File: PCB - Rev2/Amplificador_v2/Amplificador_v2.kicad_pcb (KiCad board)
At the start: 2 copper layers, 150 x 100 mm, 156 parts, among them IC1 AD817, IC2 AD817, J1 Conector alimentacion, J2 Conector alimentacion, J3 Conn_01x02_Male, J4 Conn_01x03_Male, J5 Conn_01x03_Male, J6 Screw_Terminal_01x02, J7 Conn_01x02_Male, J8 Conn_01x03_Male, J9 Screw_Terminal_01x03, Q1 BC847, Q10 BC847, Q11 BC857, Q12 BC847, Q13 2N7002, Q14 BC847, Q15 BC857, Q16 PHB27NQ10T, Q17 PHB27NQ10T, Q2 BC847, Q3 BC847, Q4 2N7002, Q5 BC857, Q6 BC847, Q7 BC847, Q8 BC857, Q9 BC857, U1 TL082, U10 LM7805_TO220, U2 LM311, U3 LM311, U4 SN74LVC2G02DCUR, U5 LM311, U6 UCC20520DWR, U7 LM7812_TO220, U8 LM7815_TO220, U9 LM7915_TO220

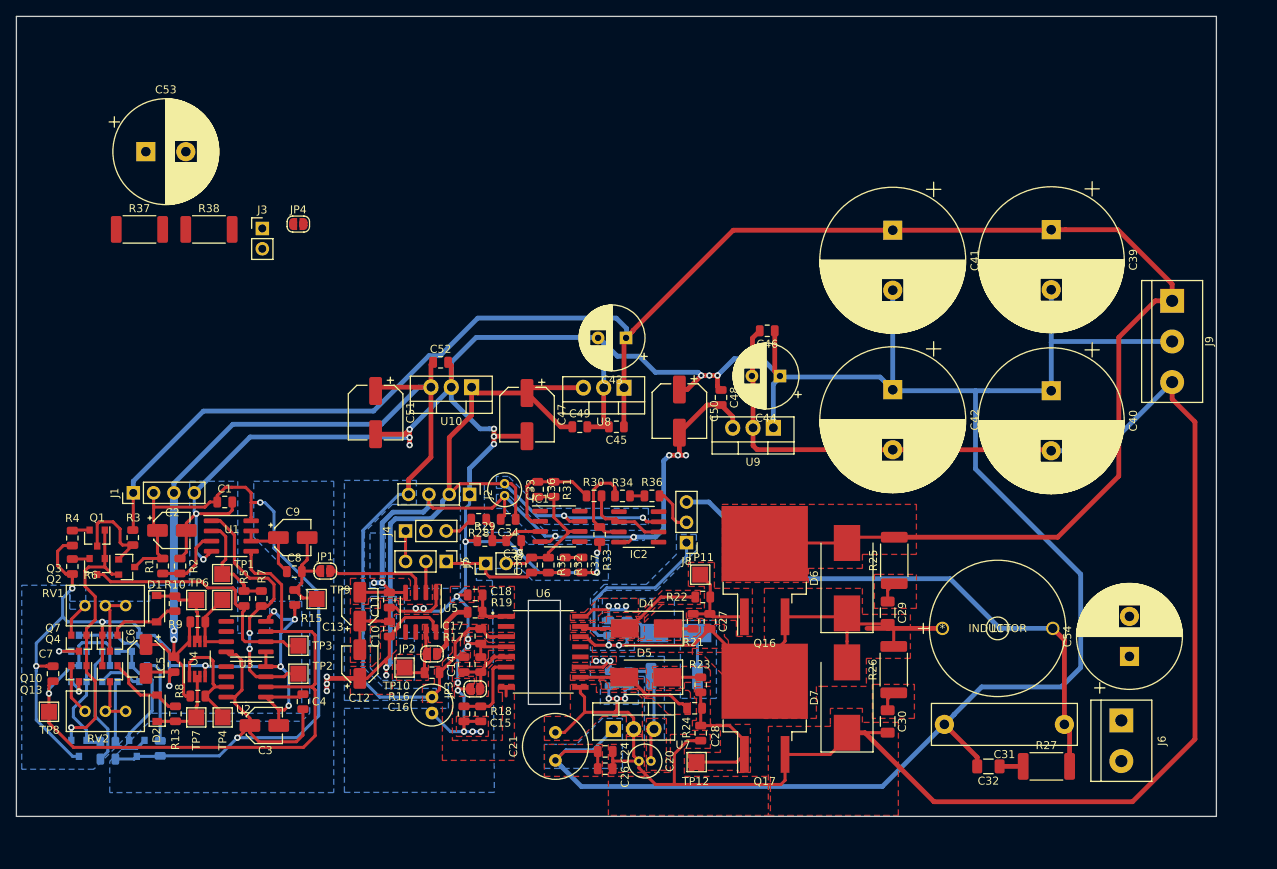
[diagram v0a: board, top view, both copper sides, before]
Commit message: Finalizada la placa v2
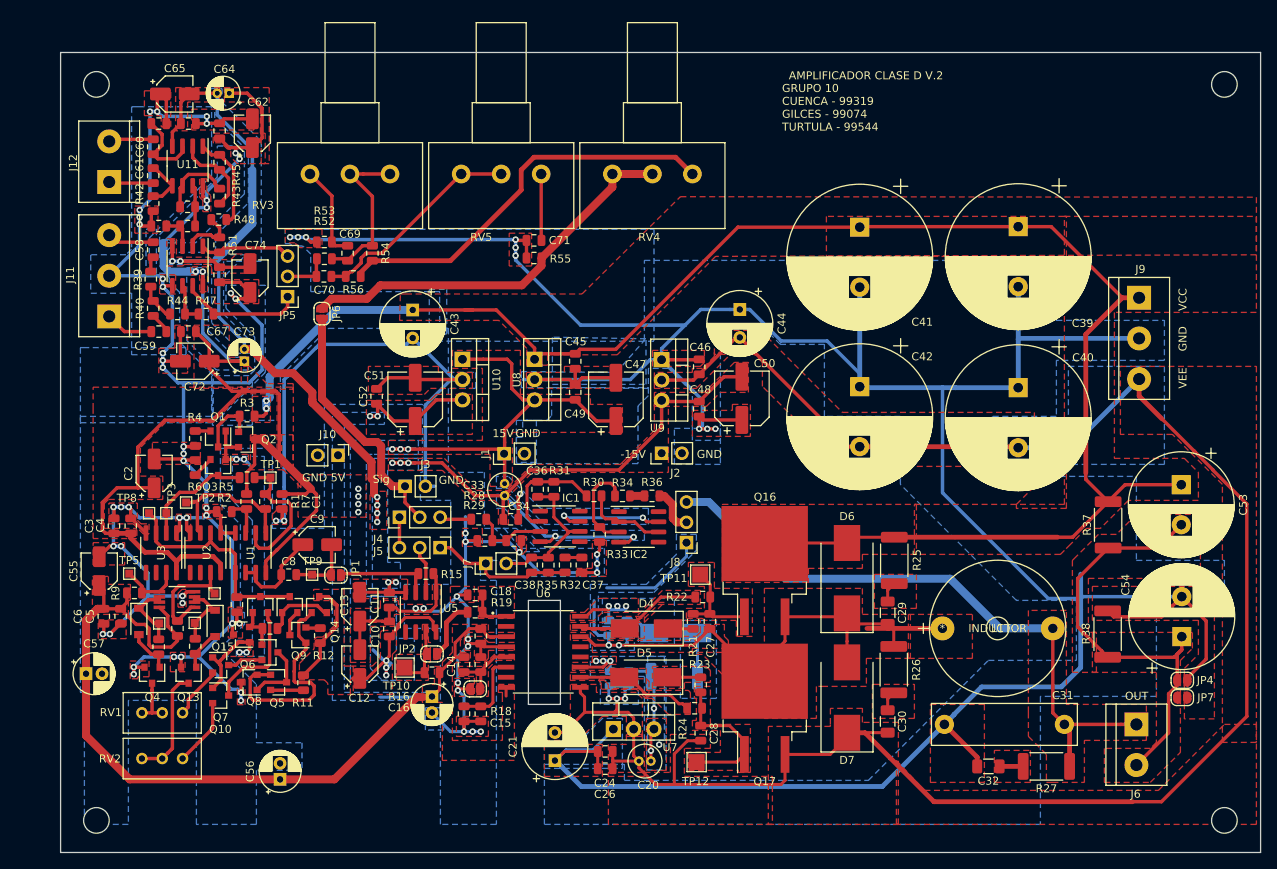
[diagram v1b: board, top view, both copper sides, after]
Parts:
- added C55: 10u, Capacitor_SMD:CP_Elec_4x5.3, F.Cu at (50.4, 144.3)
- added C56: 10u, Capacitor_THT:CP_Radial_D5.0mm_P2.00mm, F.Cu at (73.0, 170.4)
- added C57: 10u, Capacitor_THT:CP_Radial_D5.0mm_P2.00mm, F.Cu at (48.7, 157.2)
- added C58: C, Capacitor_SMD:C_0805_2012Metric, F.Cu at (57.1, 104.2)
- added C59: C, Capacitor_SMD:C_0805_2012Metric, F.Cu at (57.8, 114.4)
- added C60: C, Capacitor_SMD:C_0805_2012Metric, F.Cu at (57.1, 91.3)
- added C61: C, Capacitor_SMD:C_0805_2012Metric, F.Cu at (57.1, 94.9)
- added C62: 10u, Capacitor_SMD:CP_Elec_4x5.3, F.Cu at (69.5, 89.6)
- added C63: C, Capacitor_SMD:C_0805_2012Metric, F.Cu at (65.4, 89.3)
- added C64: 10u, Capacitor_THT:CP_Radial_D4.0mm_P1.50mm, F.Cu at (66.6, 84.6)
- added C65: 10u, Capacitor_SMD:CP_Elec_4x5.3, F.Cu at (59.8, 84.7)
- added C66: C, Capacitor_SMD:C_0805_2012Metric, F.Cu at (61.5, 88.4)
- added C67: C, Capacitor_SMD:C_0805_2012Metric, F.Cu at (61.5, 114.4)
- added C68: C, Capacitor_SMD:C_0805_2012Metric, F.Cu at (65.4, 107.3)
- added C69: C, Capacitor_SMD:C_0805_2012Metric, F.Cu at (81.4, 104.6)
- added C70: C, Capacitor_SMD:C_0805_2012Metric, F.Cu at (78.4, 107.5)
- added C71: C, Capacitor_SMD:C_0805_2012Metric, F.Cu at (104.7, 103.0)
- added C72: 10u, Capacitor_SMD:CP_Elec_4x5.3, F.Cu at (62.3, 118.1)
- added C73: 10u, Capacitor_THT:CP_Radial_D4.0mm_P1.50mm, F.Cu at (68.5, 118.1)
- added C74: 10u, Capacitor_SMD:CP_Elec_4x5.3, F.Cu at (69.2, 107.7)
- added J10: Conn_01x02_Male, Connector_PinHeader_2.54mm:PinHeader_1x02_P2.54mm_Vertical, F.Cu at (80.2, 129.9)
- added J11: Screw_Terminal_01x03, TerminalBlock:TerminalBlock_bornier-3_P5.08mm, F.Cu at (51.6, 112.5)
- added J12: Screw_Terminal_01x02, TerminalBlock:TerminalBlock_bornier-2_P5.08mm, F.Cu at (51.6, 95.7)
- added JP5: Jumper_3_Open, Connector_PinHeader_2.54mm:PinHeader_1x03_P2.54mm_Vertical, F.Cu at (73.9, 110.0)
- added JP6: Jumper_Preampli, Jumper:SolderJumper-2_P1.3mm_Open_RoundedPad1.0x1.5mm, F.Cu at (78.2, 112.2)
- added JP7: Jumper, Jumper:SolderJumper-2_P1.3mm_Open_RoundedPad1.0x1.5mm, F.Cu at (185.7, 160.1)
- added R39: R, Resistor_SMD:R_0805_2012Metric, F.Cu at (56.8, 107.8)
- added R40: R, Resistor_SMD:R_0805_2012Metric, F.Cu at (57.1, 111.5)
- added R41: R, Resistor_SMD:R_0805_2012Metric, F.Cu at (57.8, 88.4)
- added R42: R, Resistor_SMD:R_0805_2012Metric, F.Cu at (57.1, 98.4)
- added R43: R, Resistor_SMD:R_0805_2012Metric, F.Cu at (65.4, 97.5)
- added R44: R, Resistor_SMD:R_0805_2012Metric, F.Cu at (60.1, 112.2)
- added R45: R, Resistor_SMD:R_0805_2012Metric, F.Cu at (65.4, 93.2)
- added R46: R, Resistor_SMD:R_0805_2012Metric, F.Cu at (61.4, 98.8)
- added R47: R, Resistor_SMD:R_0805_2012Metric, F.Cu at (63.7, 112.2)
- added R48: R, Resistor_SMD:R_0805_2012Metric, F.Cu at (65.3, 100.4)
- added R49: R, Resistor_SMD:R_0805_2012Metric, F.Cu at (61.4, 101.2)
- added R50: R, Resistor_SMD:R_0805_2012Metric, F.Cu at (57.8, 101.2)
- added R51: R, Resistor_SMD:R_0805_2012Metric, F.Cu at (65.4, 103.6)
- added R52: R, Resistor_SMD:R_0805_2012Metric, F.Cu at (78.5, 105.3)
- added R53: R, Resistor_SMD:R_0805_2012Metric, F.Cu at (78.5, 103.2)
- added R54: R, Resistor_SMD:R_0805_2012Metric, F.Cu at (84.5, 104.6)
- added R55: R, Resistor_SMD:R_0805_2012Metric, F.Cu at (104.7, 105.2)
- added R56: R, Resistor_SMD:R_0805_2012Metric, F.Cu at (82.1, 107.5)
- added REF**: MountingHole_3.2mm_M3, MountingHole:MountingHole_3.2mm_M3, F.Cu at (50.0, 175.5)
- added REF**: MountingHole_3.2mm_M3, MountingHole:MountingHole_3.2mm_M3, F.Cu at (191.0, 175.5)
- added REF**: MountingHole_3.2mm_M3, MountingHole:MountingHole_3.2mm_M3, F.Cu at (191.0, 83.5)
- added REF**: MountingHole_3.2mm_M3, MountingHole:MountingHole_3.2mm_M3, F.Cu at (50.0, 83.5)
- added RV3: R_POT, Potentiometer_THT:Potentiometer_Alps_RK163_Single_Horizontal, F.Cu at (86.7, 94.7)
- added RV4: R_POT, Potentiometer_THT:Potentiometer_Alps_RK163_Single_Horizontal, F.Cu at (124.5, 94.7)
- added RV5: R_POT, Potentiometer_THT:Potentiometer_Alps_RK163_Single_Horizontal, F.Cu at (105.6, 94.7)
- added U11: NE5532, Package_SO:SOIC-8_3.9x4.9mm_P1.27mm, F.Cu at (61.4, 93.7)
- added U12: NE5532, Package_SO:SOIC-8_3.9x4.9mm_P1.27mm, F.Cu at (61.4, 106.2)
- C16: footprint Capacitor_THT:C_Radial_D5.0mm_H11.0mm_P2.00mm -> Capacitor_THT:CP_Radial_D5.0mm_P2.00mm
- C21: footprint Capacitor_THT:C_Radial_D8.0mm_H11.5mm_P3.50mm -> Capacitor_THT:CP_Radial_D8.0mm_P3.50mm
- C3: value 10u -> 100n; footprint Capacitor_SMD:CP_Elec_4x5.3 -> Capacitor_SMD:C_0805_2012Metric
- C6: value 10u -> 220n; footprint Capacitor_SMD:CP_Elec_4x5.3 -> Capacitor_SMD:C_0805_2012Metric
- J1, J2: value Conector alimentacion -> Conn_01x02_Male; footprint Connector_PinHeader_2.54mm:PinHeader_1x04_P2.54mm_Vertical -> Connector_PinHeader_2.54mm:PinHeader_1x02_P2.54mm_Vertical
- Q11, Q12, Q14, Q15, Q5, Q6, Q8, Q9, R11, R12, R14: moved to F.Cu
- TP1, TP2, TP3, TP4, TP5, TP6, TP7, TP8, TP9: footprint TestPoint:TestPoint_Pad_2.0x2.0mm -> TestPoint:TestPoint_Pad_1.0x1.0mm
- moved C53 136.0 mm to (185.6, 133.5), turned to 270 degrees
- moved R37 126.6 mm to (176.5, 138.6), turned to 90 degrees
- moved JP4 124.3 mm to (185.7, 158.0), turned to 180 degrees
- moved R38 123.2 mm to (176.4, 152.2), turned to 270 degrees
- moved J1 46.6 mm to (101.0, 129.7)
- moved J3 36.8 mm to (88.6, 133.7), turned to 90 degrees
- moved C3 31.2 mm to (52.2, 138.7), turned to 90 degrees
- moved C4 30.8 mm to (54.3, 138.7)
- moved Q14 29.0 mm to (77.9, 148.5), turned to 90 degrees
- moved TP8 27.8 mm to (56.6, 137.1), turned to 270 degrees
- moved C43 26.9 mm to (89.5, 111.7), turned to 270 degrees
- moved R11 26.2 mm to (75.9, 158.3), turned to 270 degrees
- moved TP2 25.6 mm to (61.2, 135.8), turned to 270 degrees
- moved Q15 24.8 mm to (68.1, 152.3), turned to 180 degrees
- moved R14 24.8 mm to (71.7, 151.5)
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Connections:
- J1 pad 1: VCC -> +15V
- J1 pad 2: +15V -> GND
- J2 pad 1: GND -> -15V
- J2 pad 2: +15V -> GND
- R15 pad 1: Net-(C8-Pad2) -> Vtriang
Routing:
- net GND: track 603.4 -> 813.2 mm, vias 34 -> 67
- net -15V: track 90.4 -> 184.8 mm, vias 7 -> 13
- net /Vtriang_off: track 92.9 -> 28.1 mm, vias 1 -> 0
- net Net-(C53-Pad2): track 0.00 -> 55.8 mm
- net /Filter_out: track 0.00 -> 50.3 mm
- net Net-(JP6-Pad1): track 0.00 -> 49.8 mm
- net +15V: track 239.8 -> 279.2 mm, vias 9 -> 19
- net Signal_in: track 0.00 -> 31.7 mm
- net Net-(C70-Pad2): track 0.00 -> 26.9 mm
- net VCC: track 241.6 -> 217.1 mm, vias 0 -> 2
- net +5V: track 152.6 -> 129.8 mm
- net Net-(C69-Pad2): track 0.00 -> 21.1 mm
- net /U-: track 32.5 -> 14.2 mm
- net Net-(JP5-Pad1): track 0.00 -> 15.9 mm
- net /U+: track 32.2 -> 18.4 mm, vias 2 -> 0
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- added copper zone on F.Cu, net Net-(C32-Pad1)
- added copper zone on F.Cu, net Net-(C53-Pad2)
- added copper zone on B.Cu, net Net-(Q1-Pad1)
- added copper zone on F.Cu, net Net-(Q1-Pad1)
- added copper zone on F.Cu, net VOUT
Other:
- outline, holes or cut-outs redrawn
- board text added: "-15V"
- board text added: "15V"
- board text added: "5V"
- board text added: "AMPLIFICADOR CLASE D V.2"
- board text added: "GND"
- board text added: "GRUPO 10 CUENCA - 99319 GILCES - 99074 TURTULA - 99544"
- board text added: "OUT"
- board text added: "Sig"
- board text added: "VCC"
- board text added: "VEE"
